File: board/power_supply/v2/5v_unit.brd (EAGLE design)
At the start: 25.1 x 51.4 mm, 12 parts

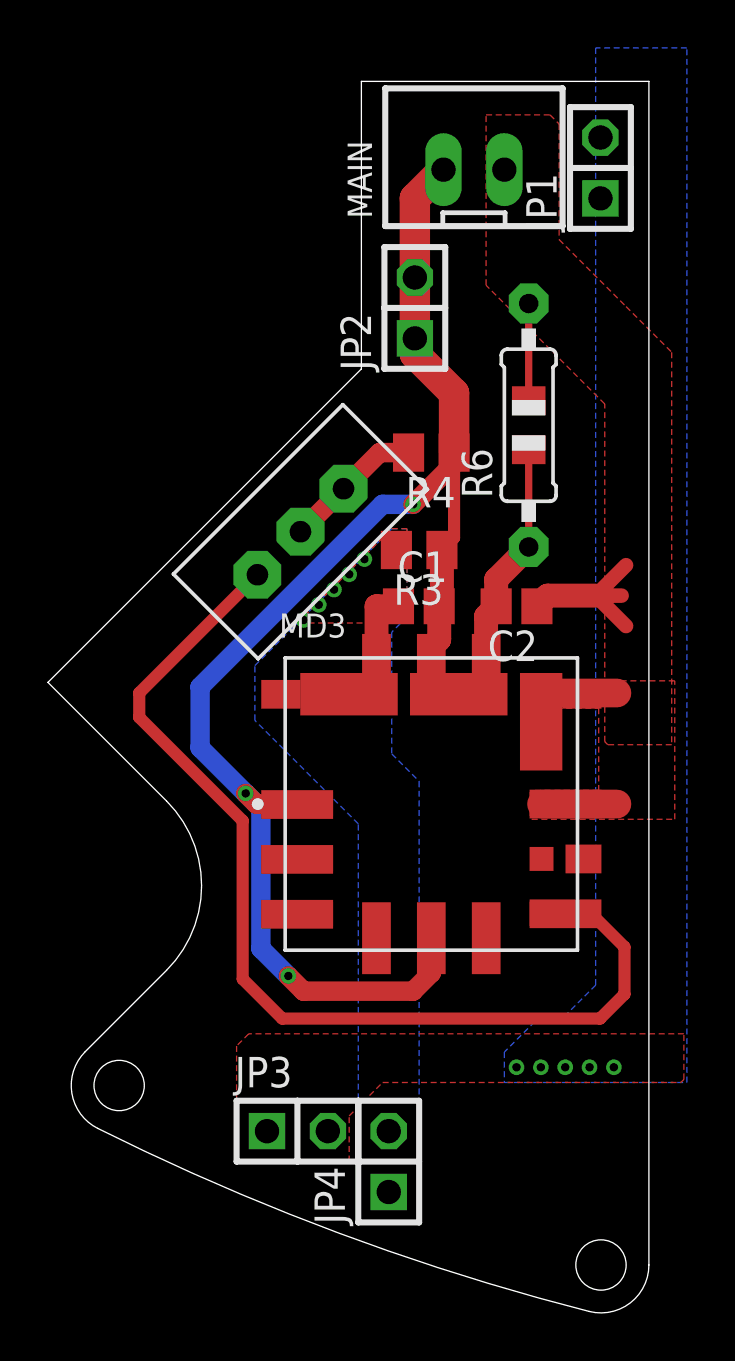
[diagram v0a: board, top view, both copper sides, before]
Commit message: change dimention & check DRC
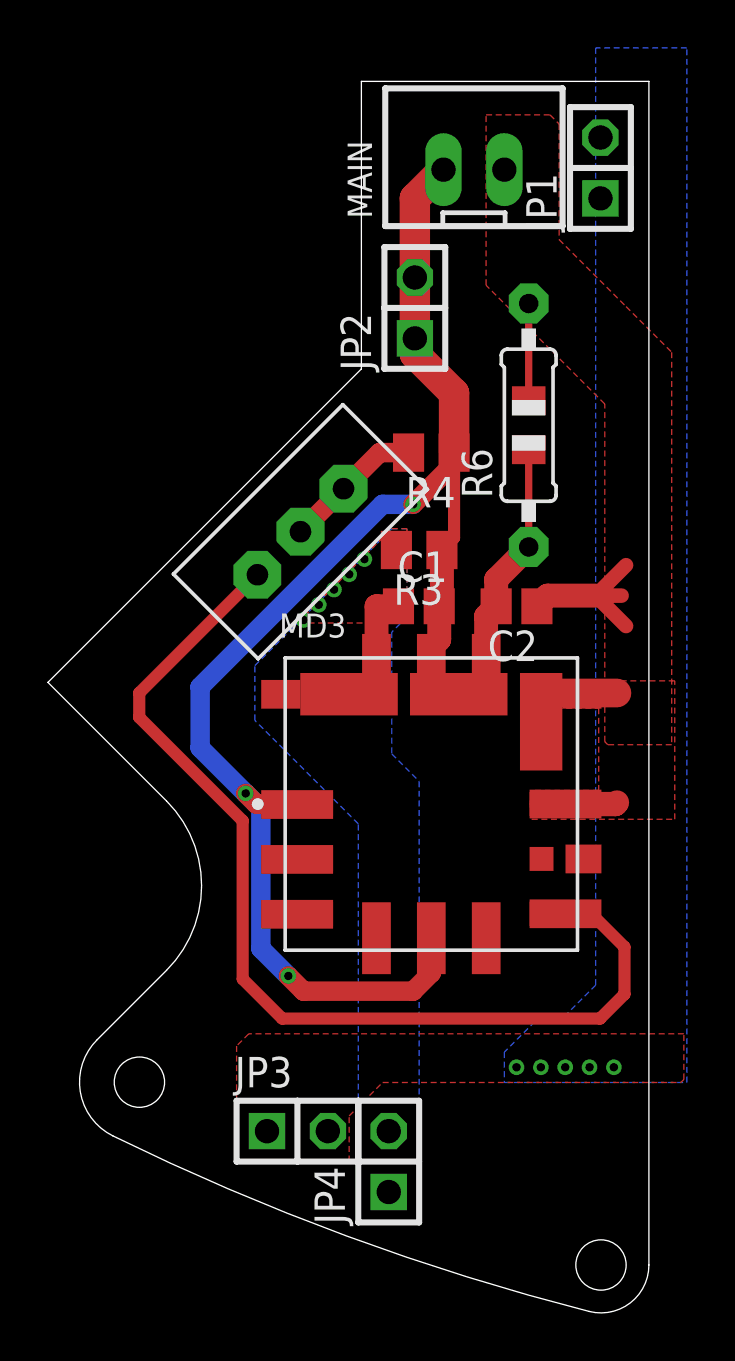
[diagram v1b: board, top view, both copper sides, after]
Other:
- outline, holes or cut-outs redrawn
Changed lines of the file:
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@@
 <drawing>
 <settings>
-<setting alwaysvectorfont="yes"/>
+<setting alwaysvectorfont="no"/>
 <setting verticaltext="up"/>
 </settings>
@@
 <fusionsync huburn="a.cGVyc29uYWw6dWUyYjhiNWJj" projecturn="a.cGVyc29uYWw6dWUyYjhiNWJjIzIwMjIwNDE2NTE3MzEzNjU2" f3durn="urn:adsk.wipprod:dm.lineage:J4KWdsV-RwmCOziydWyP5A" pcbguid="" lastpulledtime="" lastsyncedchangeguid="" latestrevisionid="46676070-bb23-41f3-9839-3d353bdf0556" lastsyncedrevisionid="46676070-bb23-41f3-9839-3d353bdf0556" lastboardhashguid="7af40513-0a80-27c1-dc80-51a4a12e53d5" lastpushedtime="2022-10-04T02:11:47Z" linktopcb3d="true"/>
 <plain>
-<circle x="2.972209375" y="10.03331875" radius="1.05" width="0.001" layer="20"/>
 <circle x="23.083259375" y="2.542159375" radius="1.05" width="0.001" layer="20"/>
-<wire x1="1.558" y1="11.44753125" x2="2.07891875" y2="8.2439" width="0.001" layer="20" curve="108.47"/>
-<wire x1="2.07891875" y1="8.2439" x2="22.58841875" y2="0.60435" width="0.001" layer="20" curve="12.2"/>
-<wire x1="22.58841875" y1="0.60435" x2="25.083259375" y2="2.542159375" width="0.001" layer="20" curve="104.32"/>
-<wire x1="25.083259375" y1="2.542159375" x2="25.083259375" y2="51.943359375" width="0.001" layer="20"/>
+<wire x1="25.083259375" y1="51.943359375" x2="25.083259375" y2="2.542159375" width="0.001" layer="20"/>
 <wire x1="25.083259375" y1="51.943359375" x2="13.083259375" y2="51.943359375" width="0.001" layer="20"/>
 <wire x1="13.083259375" y1="51.943359375" x2="13.083259375" y2="39.943359375" width="0.001" layer="20"/>
 <wire x1="13.083259375" y1="39.943359375" x2="0" y2="26.8601" width="0.001" layer="20"/>
 <wire x1="0" y1="26.8601" x2="4.94975" y2="21.91035" width="0.001" layer="20"/>
-<wire x1="4.94975" y1="21.91035" x2="4.94975" y2="14.83928125" width="0.001" layer="20" curve="-90"/>
-<wire x1="4.94975" y1="14.83928125" x2="1.558" y2="11.44753125" width="0.001" layer="20"/>
+<wire x1="4.94975" y1="14.83928125" x2="4.94975" y2="21.91035" width="0.001" layer="20" curve="90"/>
+<wire x1="2.706109375" y1="7.933459375" x2="22.58841875" y2="0.60435" width="0.001" layer="20" curve="11.808321"/>
+<wire x1="22.58841875" y1="0.60435" x2="25.083259375" y2="2.542159375" width="0.001" layer="20" curve="104.324739"/>
+<circle x="3.818409375" y="10.17241875" radius="1.05" width="0.001" layer="20"/>
+<wire x1="2.05935" y1="11.948890625" x2="2.706109375" y2="7.933459375" width="0.001" layer="20" curve="108.864352"/>
+<wire x1="4.94975" y1="14.83928125" x2="2.05935" y2="11.948890625" width="0.001" layer="20"/>
 </plain>
 <attributes>
@@
 </class>
 </classes>
-<designrules name="Elecrow_2-layer_PCB_eagle_rule *">
+<designrules name="Elecrow_2-layer_PCB_eagle_rule">
 <description language="de">&lt;b&gt;EAGLE Design Rules&lt;/b&gt;
 &lt;p&gt;
@@
 <param name="layerSetup" value="(1*16)"/>
 <param name="mtCopper" value="0.035mm 0.035mm 0.035mm 0.035mm 0.035mm 0.035mm 0.035mm 0.035mm 0.035mm 0.035mm 0.035mm 0.035mm 0.035mm 0.035mm 0.035mm 0.035mm"/>
-<param name="mtIsolate" value="1.2mm 1.2mm 0.2mm 0.15mm 0.2mm 0.15mm 0.2mm 0.15mm 0.2mm 0.15mm 0.2mm 0.15mm 0.2mm 0.15mm 0.2mm"/>
+<param name="mtIsolate" value="1.6mm 1.2mm 0.2mm 0.15mm 0.2mm 0.15mm 0.2mm 0.15mm 0.2mm 0.15mm 0.2mm 0.15mm 0.2mm 0.15mm 0.2mm"/>
 <param name="mdWireWire" value="6mil"/>
 <param name="mdWirePad" value="6mil"/>
@@
 <vertex x="20.193" y="22.352"/>
 </polygon>
-<wire x1="20.587" y1="25.2155" x2="20.587" y2="25.4" width="1.27" layer="1"/>
-<wire x1="20.602" y1="21.7805" x2="23.749" y2="21.7805" width="1.2" layer="1"/>
 <polygon width="0.254" layer="1" spacing="0.4064" thermals="no">
 <vertex x="18.288" y="50.546"/>
@@
 <wire x1="22.86" y1="30.48" x2="24.13" y2="31.75" width="0.6096" layer="1"/>
 <wire x1="22.86" y1="30.48" x2="24.13" y2="29.21" width="0.6096" layer="1"/>
+<wire x1="20.602" y1="21.7805" x2="23.6855" y2="21.7805" width="1.016" layer="1"/>
+<wire x1="23.6855" y1="21.7805" x2="23.749" y2="21.844" width="1.016" layer="1"/>
 </signal>
 <signal name="N$9">
